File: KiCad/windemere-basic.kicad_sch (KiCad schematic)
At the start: 64 parts, among them J1 Barrel_Jack, J2 Connector, J3 A_40-LC-TT, J4 A_28-LC-TT, J5 A_40-LC-TT, J6 A_28-LC-TT, SW1 Reset Button, U1 L7805, U2 74HC00, U3 WD65C02, U4 28C256, U5 62256, U6 WD65C22, U7 MM74C922, U8 HD44780U, U9 MCP102-475, X1 1MHz

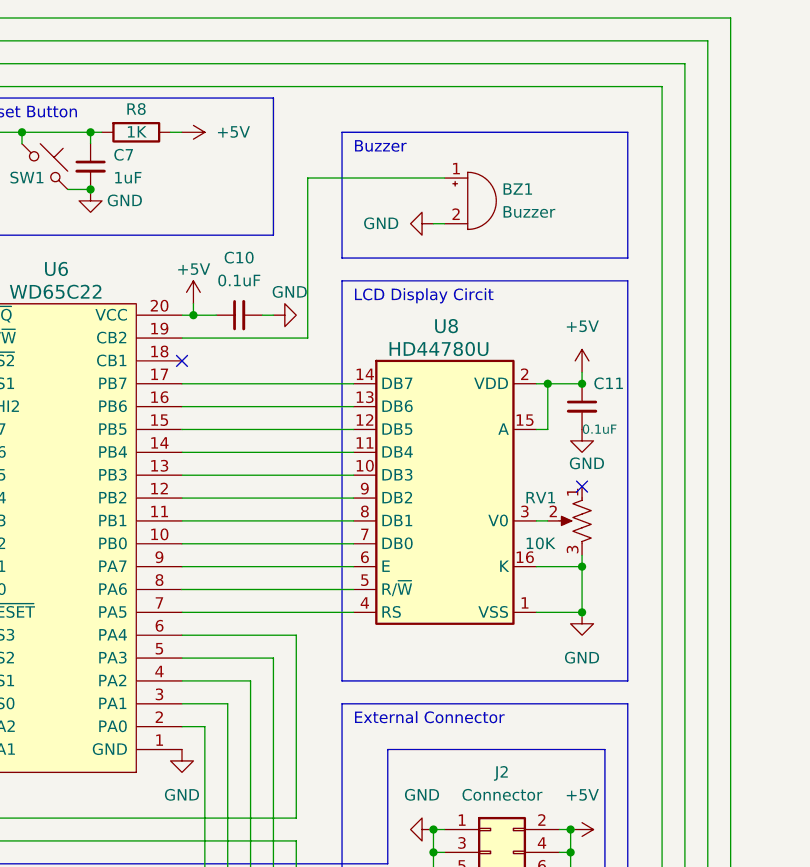
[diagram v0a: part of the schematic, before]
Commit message: Update windemere-basic.kicad_sch
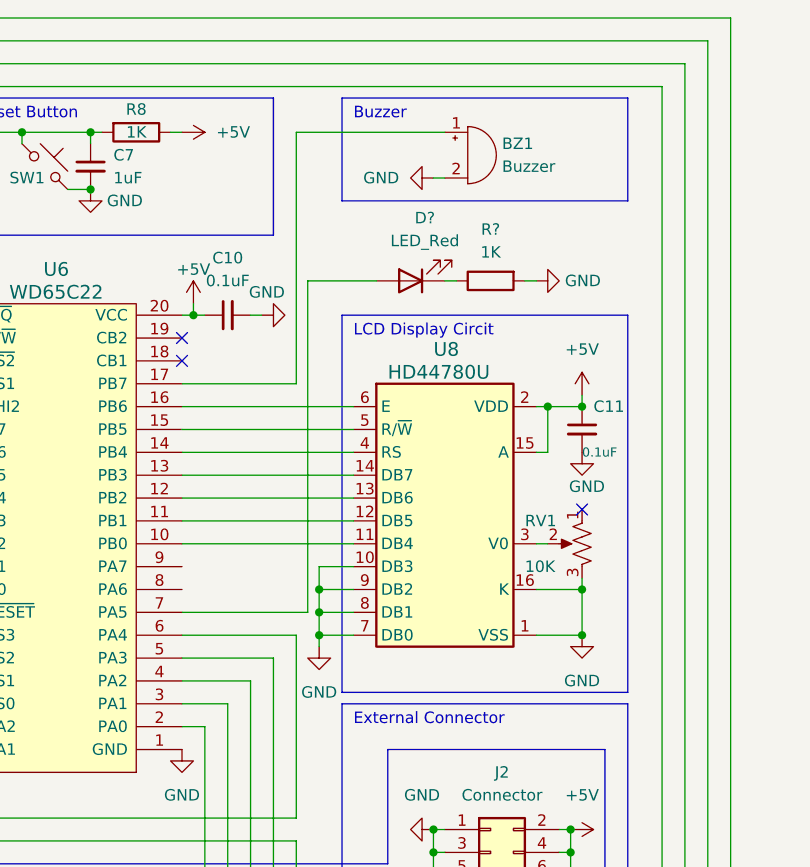
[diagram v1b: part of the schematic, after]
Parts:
- added D?: LED_Red, LED_THT:LED_D5.0mm, symbol Device:LED
- added R?: 1K, Resistor_THT:R_Axial_DIN0207_L6.3mm_D2.5mm_P10.16mm_Horizontal, symbol Device:R
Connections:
- net GND: now also U8.10 (DB3), U8.7 (DB0), U8.8 (DB1), U8.9 (DB2), R?.2
- net at BZ1.1 (-): now also U6.17 (PB7); no longer U6.19 (CB2)
- net at U6.10 (PB0): now also U8.11 (DB4); no longer U8.7 (DB0)
- net at U6.11 (PB1): now also U8.12 (DB5); no longer U8.8 (DB1)
- net at U6.12 (PB2): now also U8.13 (DB6); no longer U8.9 (DB2)
- net at U6.13 (PB3): now also U8.14 (DB7); no longer U8.10 (DB3)
- net at U6.14 (PB4): now also U8.4 (RS); no longer U8.11 (DB4)
- net at U6.15 (PB5): now also U8.5 (R/~{W}); no longer U8.12 (DB5)
- net at U6.16 (PB6): now also U8.6 (E); no longer U8.13 (DB6)
- net at U6.7 (PA5): now also D?.2 (A); no longer U8.4 (RS)
- net at U6.8 (PA6): no longer U8.5 (R/~{W})
- net at U6.9 (PA7): no longer U8.6 (E)
- new net: D?.1 (K), R?.1
- no-connect marks 145 -> 146
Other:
- moved on the sheet: BZ1, C10, C11, RV1, U8
